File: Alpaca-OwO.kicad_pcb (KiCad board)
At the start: 4 copper layers, 100 x 45 mm, 43 parts, among them J1 SWD, J2 PS360 ST1, J3 PS360 ST2, J4 Stick, J5 USB_B, J6 Pwny Pr0t, J7 I2C Quick connect, Q1 CJL3415, SW1 Reset, SW2 I2C Pullup, SW3 BootSel, U1 AMS1117-3.3, U2 RP2040, U3 W25Q32JVSS, Y1 12MHz

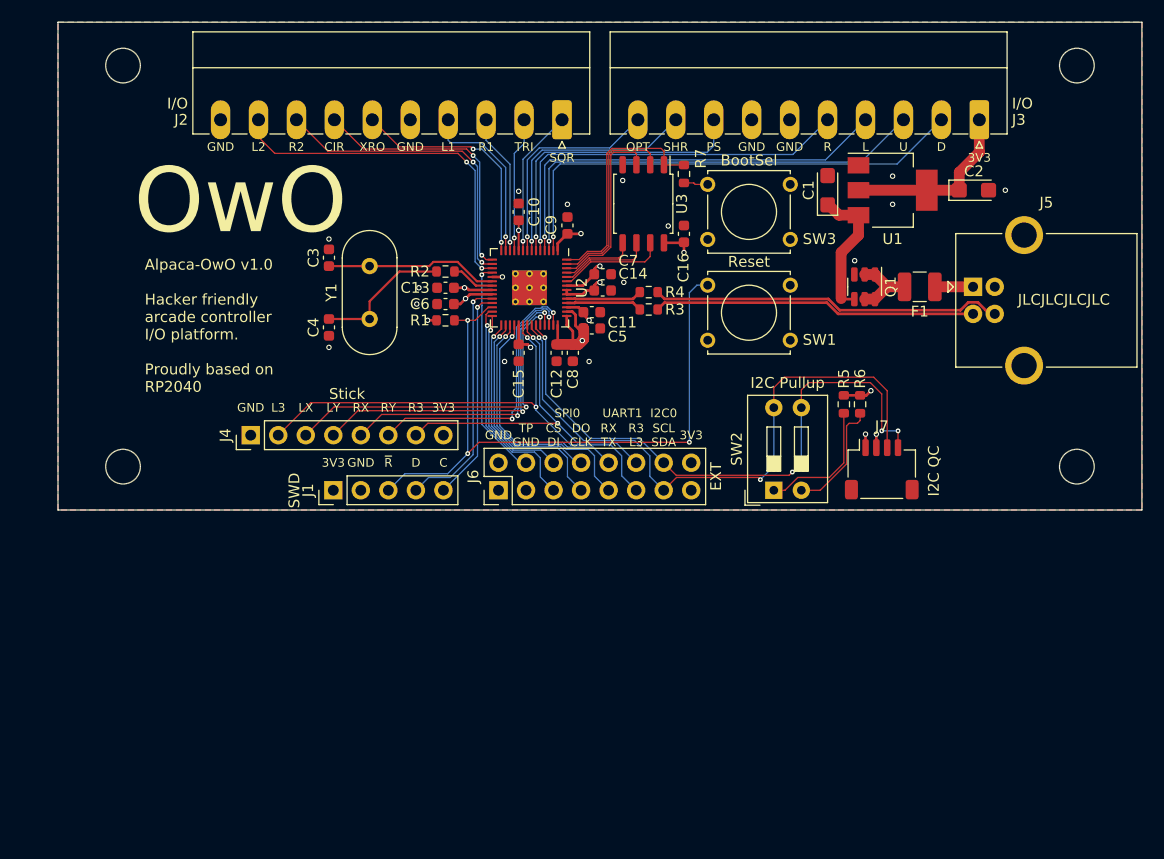
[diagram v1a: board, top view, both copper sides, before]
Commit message: V1.01 rework.
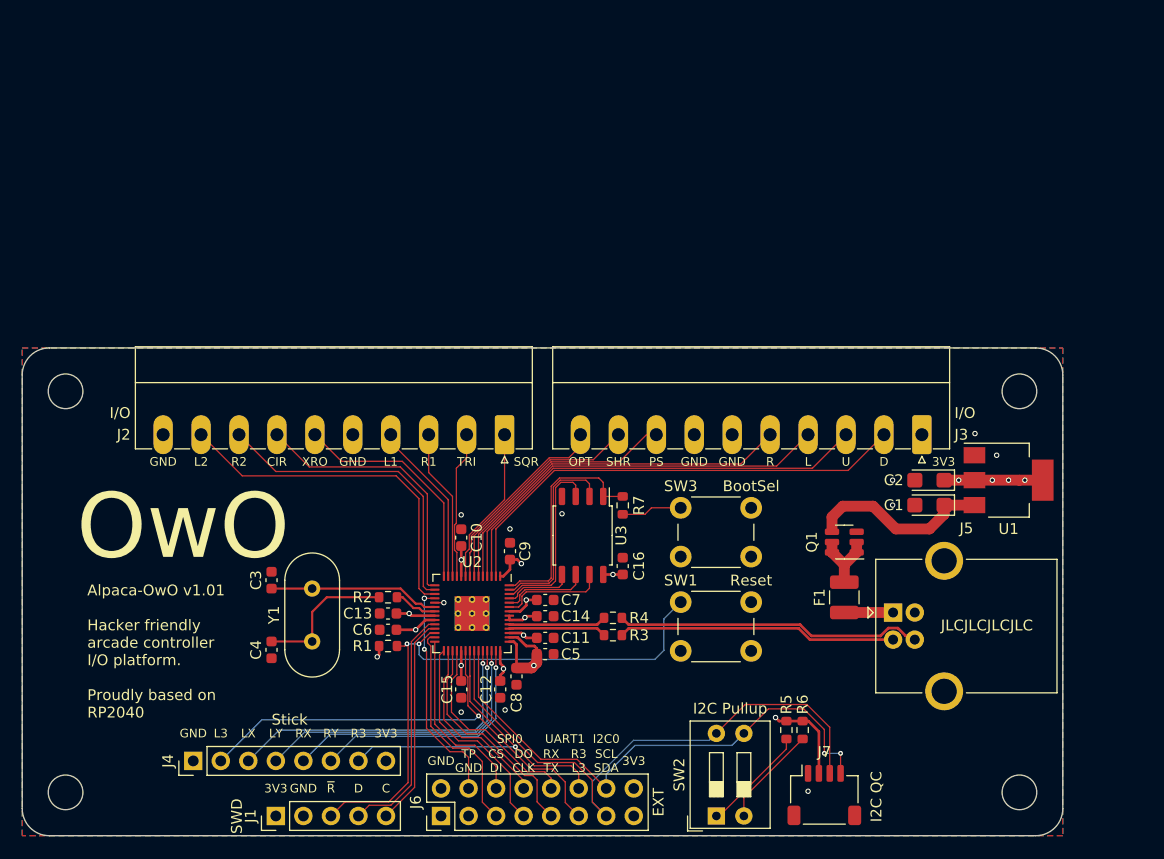
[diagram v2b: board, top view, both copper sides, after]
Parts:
- SW1, SW3: footprint Button_Switch_THT:SW_Tactile_Straight_KSA0Axx1LFTR -> Button_Switch_THT:SW_PUSH_6mm
- moved C15 31.5 mm to (148.2, 109.5)
- moved C12 31.5 mm to (151.8, 109.5)
- moved C16 31.2 mm to (163.1, 98.2)
- moved U3 31.1 mm to (159.4, 95.3)
- moved R7 31.1 mm to (163.1, 92.6)
- moved J5 30.9 mm to (188.0, 102.5)
- moved C1 30.5 mm to (191.4, 92.5), turned to 180 degrees
- moved J4 30.5 mm to (123.5, 116.2)
- moved C10 30.5 mm to (148.2, 95.5)
- moved C13 30.5 mm to (141.4, 102.5)
- moved C14 30.5 mm to (155.9, 102.8)
- moved C6 30.5 mm to (141.4, 104.0)
- moved C7 30.5 mm to (155.9, 101.3)
- moved C9 30.5 mm to (152.7, 96.8)
- moved H1 30.5 mm to (111.7, 119.0)
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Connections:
- SW1 pad 1: GND -> /~{RESET}
- SW1 pad 2: /~{RESET} -> GND
- SW3 pad 1: GND -> Net-(R7-Pad1)
- SW3 pad 2: Net-(R7-Pad1) -> GND
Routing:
- net +1V1: track 27.4 -> 9.90 mm
- net /~{RESET}: track 61.3 -> 54.4 mm, vias 3 -> 2
- net /I2C0_SCL: track 54.9 -> 49.8 mm, vias 4 -> 2
- net Net-(C1-Pad1): track 12.7 -> 17.2 mm
- net /USB_D-: track 29.8 -> 25.7 mm
- net +3V3: track 51.8 -> 48.2 mm, vias 10 -> 14
- net /USB_D+: track 32.0 -> 28.5 mm
- net /KEY_PS: track 27.6 -> 24.1 mm, vias 1 -> 0
- net Net-(R7-Pad1): track 2.25 -> 5.60 mm
- net /STK_RY: track 26.2 -> 23.1 mm, vias 2 -> 1
- net /STK_RX: track 28.3 -> 25.3 mm, vias 2 -> 1
- net /UART1_TX: track 23.7 -> 20.7 mm, vias 1 -> 0
- net /UART1_RX: track 21.3 -> 18.5 mm, vias 1 -> 0
- net /STK_LY: track 30.1 -> 27.5 mm, vias 2 -> 1
- net /KEY_SHR: track 23.2 -> 20.9 mm, vias 1 -> 0
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- added copper zone on In2.Cu, net +1V1
- added copper zone on In1.Cu, net GND
- removed copper zone on In1.Cu, net +3V3
- removed copper zone on In2.Cu, net GND
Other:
- board size 100 x 45 mm -> 96 x 45 mm
- board text added: "Alpaca-OwO v1.01 Hacker friendly arcade controller I/O platform. Proudly based on RP2040"
- board text removed: "Alpaca-OwO v1.0 Hacker friendly arcade controller I/O platform. Proudly based on RP2040"
